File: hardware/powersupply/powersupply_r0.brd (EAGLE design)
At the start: 160 x 100 mm, 20 parts

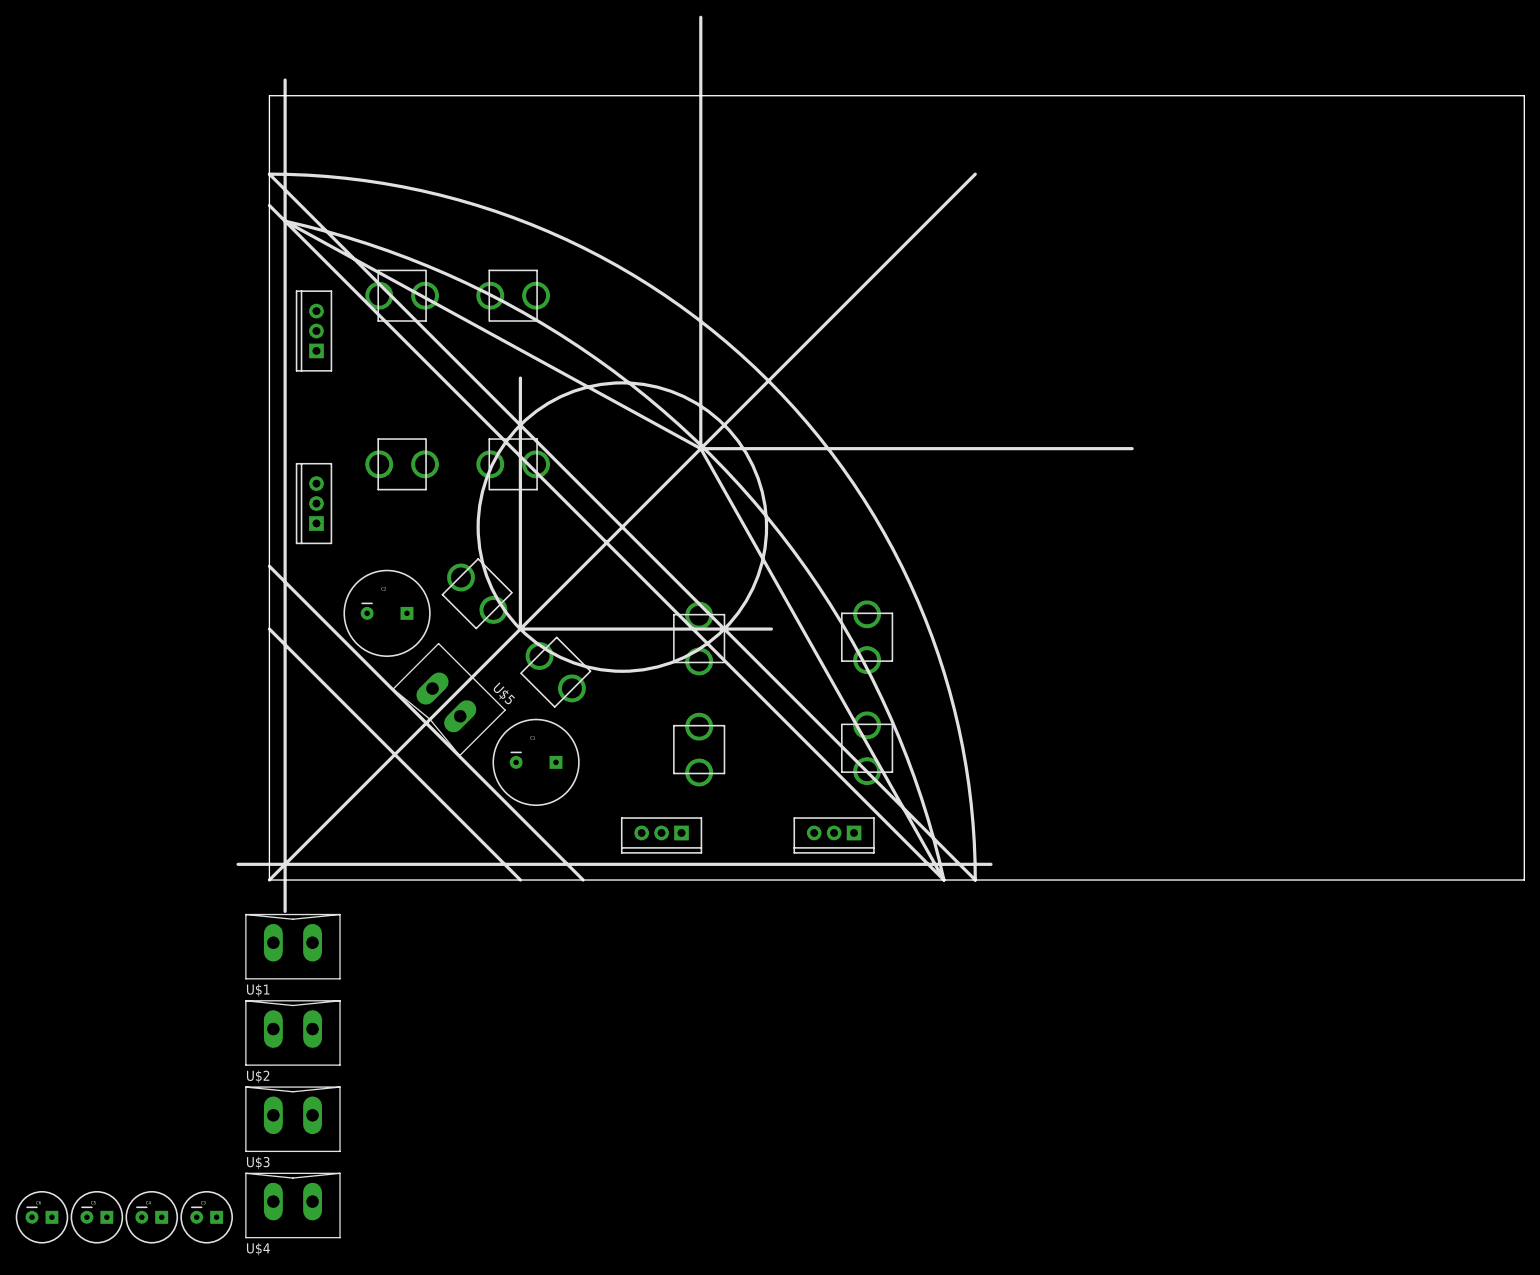
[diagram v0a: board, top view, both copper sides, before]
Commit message: component layout complete
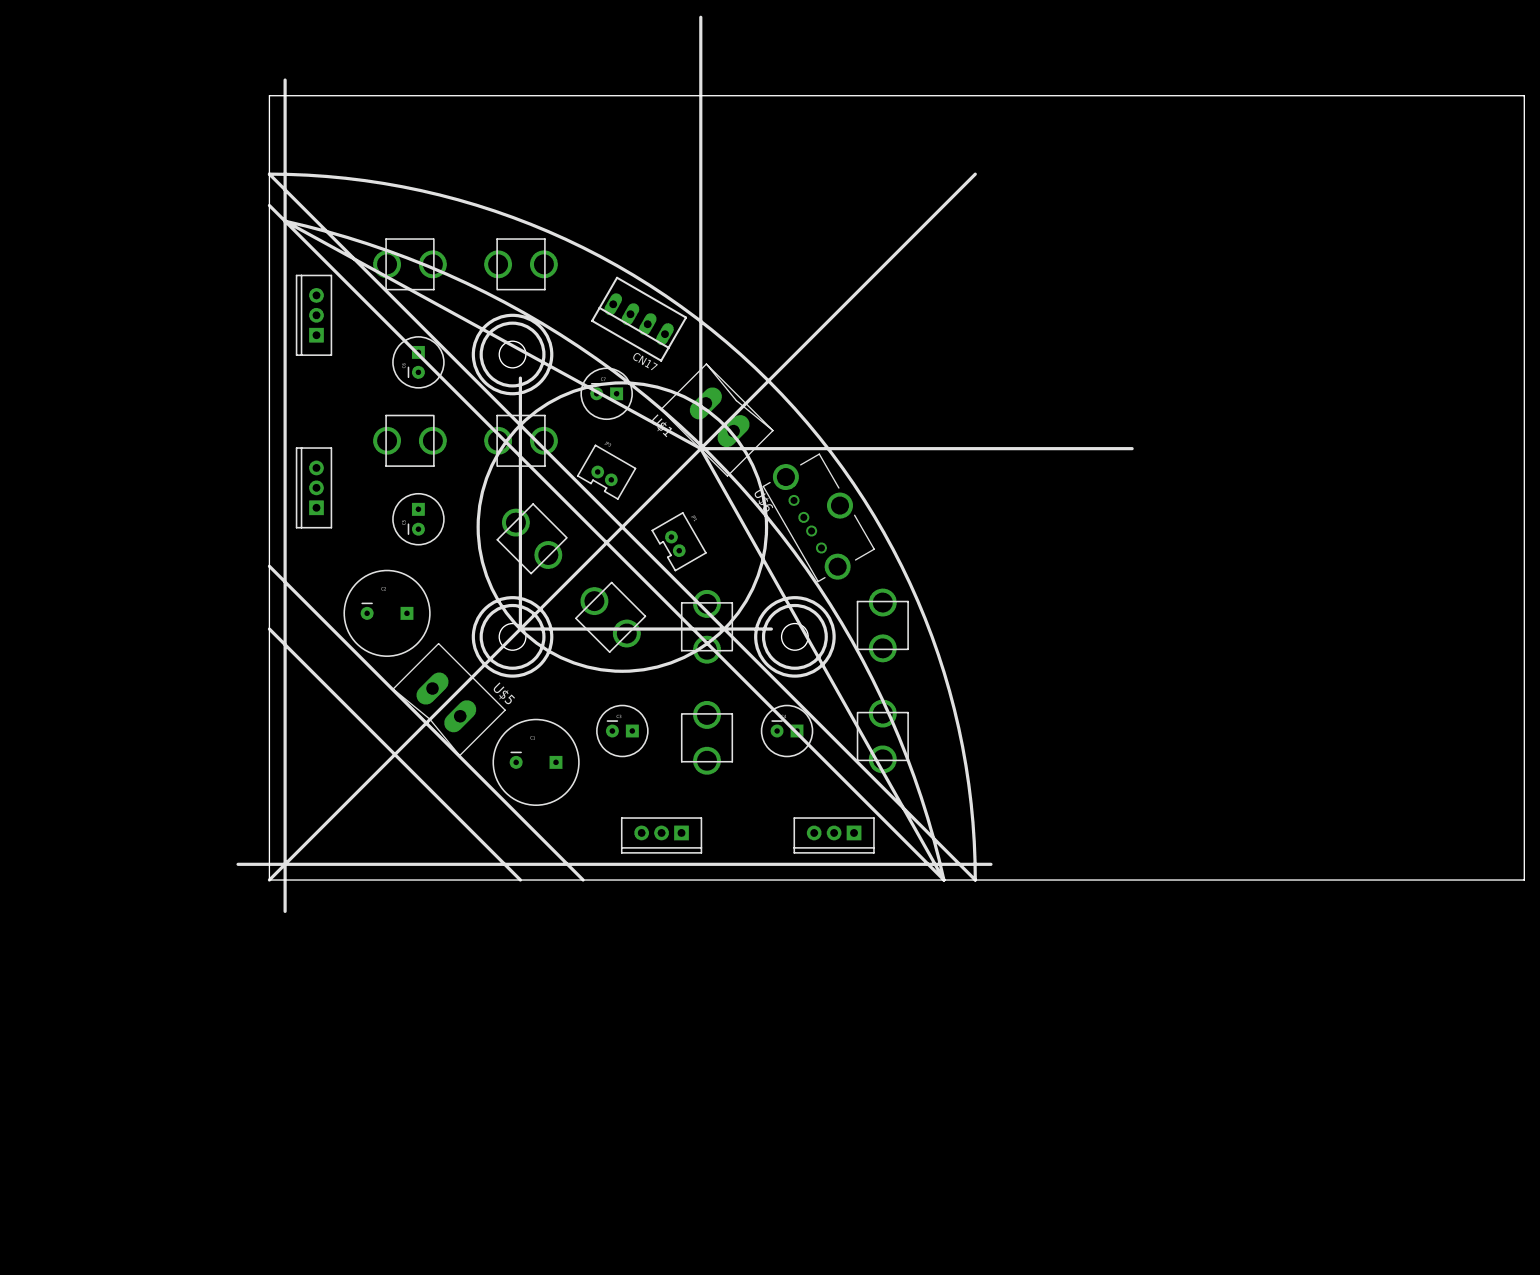
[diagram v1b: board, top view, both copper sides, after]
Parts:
- removed U$2, U$3, U$4: SCREWTERMINAL-2PIN, openct:SCREWTERMINAL-2PIN
- added C7: (no value), SparkFun-Passives:CPOL-RADIAL-100UF-25V
- added CN17: 22-23-2041, con-molex:22-23-2041
- added JP1, JP3: M02JST-PTH-VERT, SparkFun-Connectors:JST-2-PTH-VERT
- added U$6: CON-USB, openct:MOLEX-USB-105057-0001
- moved C6 119.1 mm to (19.0, 66.0), turned to 90 degrees
- moved C4 102.0 mm to (66.0, 19.0)
- moved C5 98.0 mm to (19.0, 46.0), turned to 90 degrees
- moved U$1 86.3 mm to (57.4, 59.0), turned to 315 degrees
- moved C3 81.6 mm to (45.0, 19.0)
- moved F5 9.90 mm to (38.5, 38.5)
- moved F4 4.12 mm to (25.0, 78.5), turned to 270 degrees
- moved F3 3.16 mm to (25.0, 56.0), turned to 270 degrees
- moved F2 2.50 mm to (78.2, 25.4)
- moved IC3 2.00 mm to (6.00, 50.0)
- moved IC4 2.00 mm to (6.00, 72.0)
- moved F1 1.80 mm to (55.8, 25.2)
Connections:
- new net GND: C3.2, C4.2, C5.2, C6.2, C7.2, CN17.2, CN17.3, IC1.GND, IC2.GND, IC3.GND, IC4.GND, U$1.2
- new net N$1: C3.1, F1.1, IC1.OUT
- new net N$2: C4.1, F2.1, IC2.OUT
- new net N$3: C5.1, F3.1, IC3.OUT
- new net N$4: C6.1, F4.1, IC4.OUT
- new net N$5: CN17.4, F4.3
- new net VBIAS: C7.1, CN17.1, U$1.1
